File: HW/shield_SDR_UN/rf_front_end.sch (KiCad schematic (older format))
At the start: 73 parts, among them P1 GSG-RF-CONN, P2 GSG-RF-CONN, Q1 MOSFET_P, T1 BALUN, T2 BALUN, U1 MAX2830, U2 SI5351C, U3 MAX5864, X1 GSG-XTAL4PIN

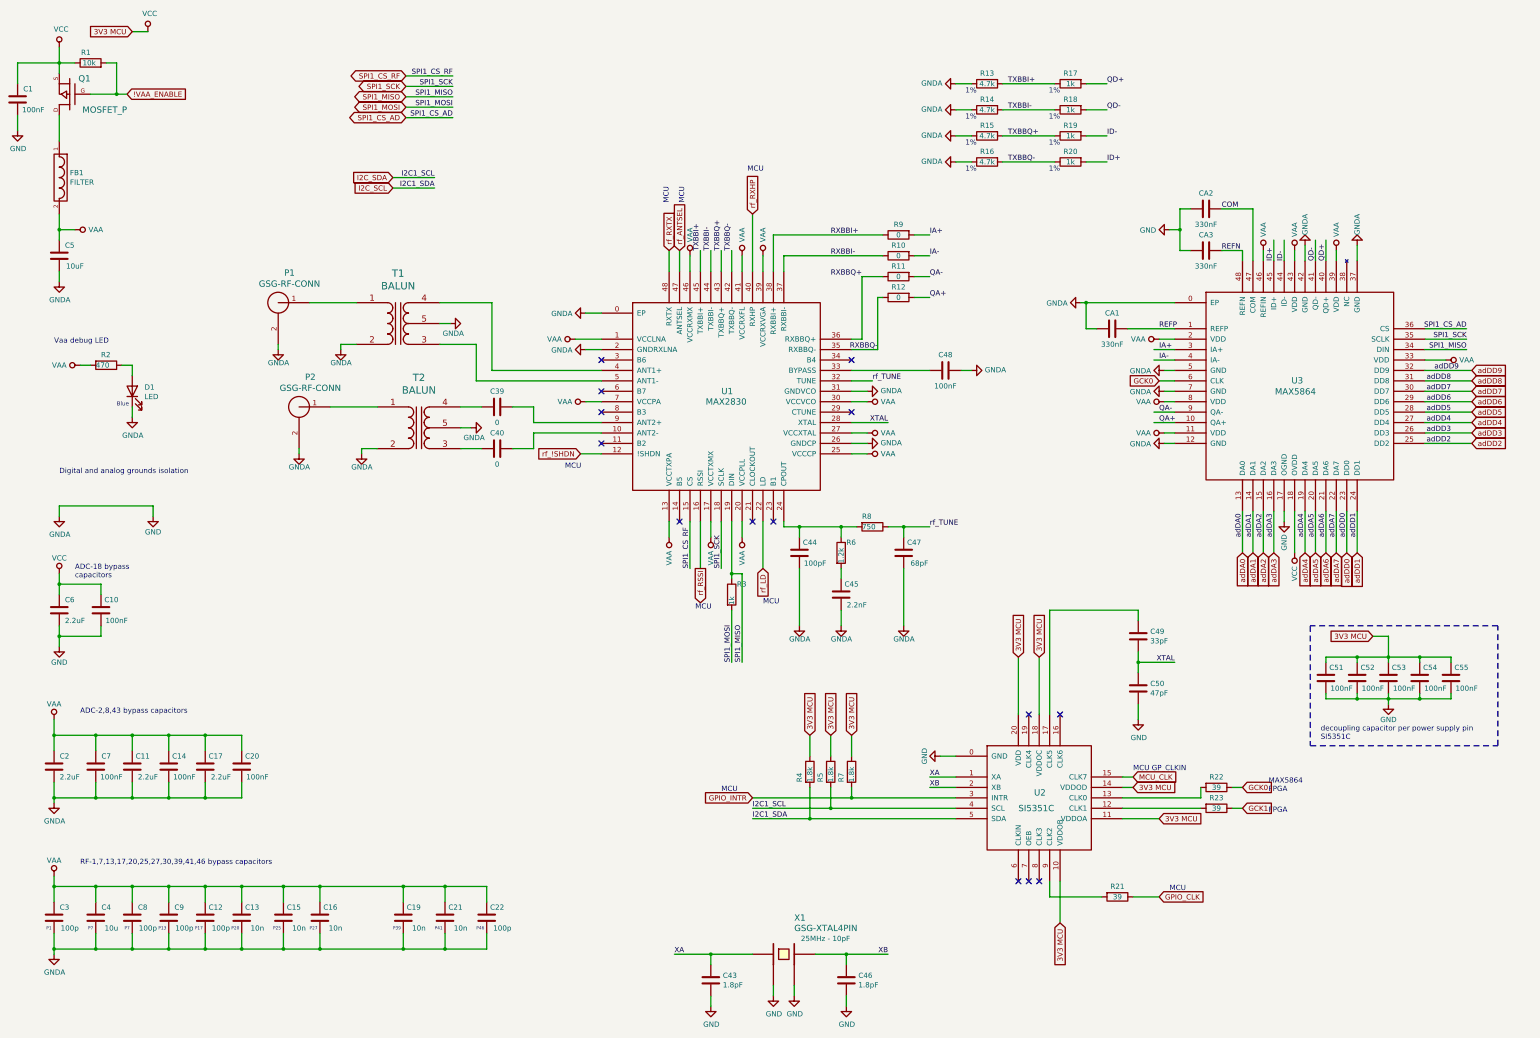
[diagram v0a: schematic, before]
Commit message: PCB route V4
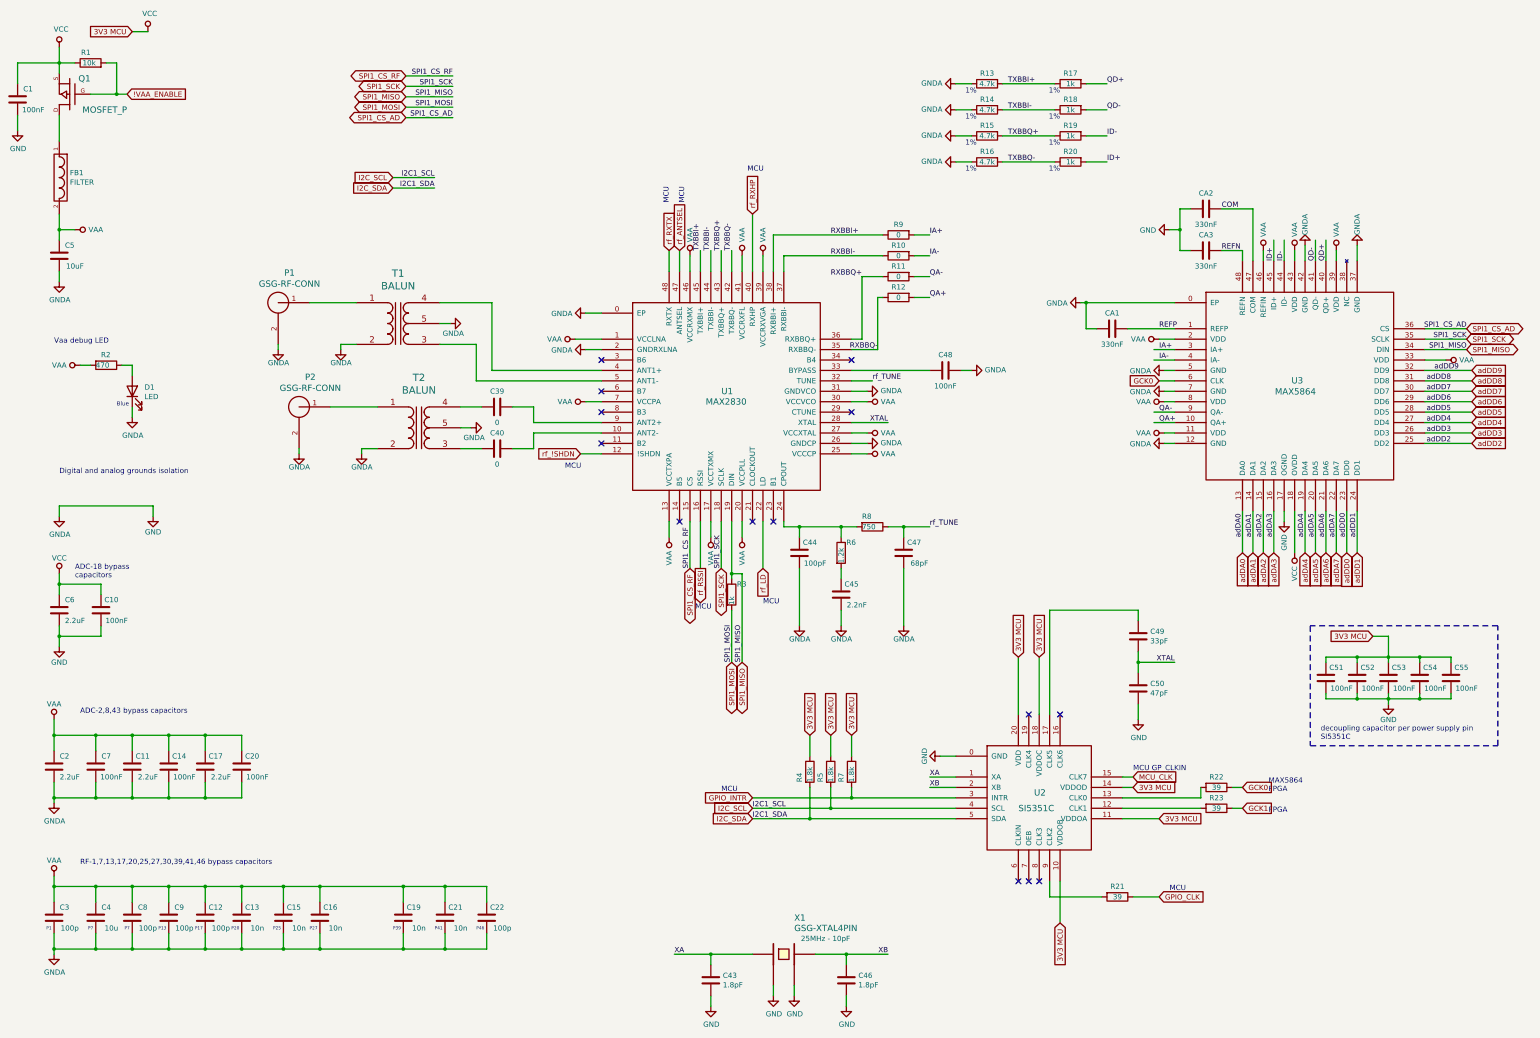
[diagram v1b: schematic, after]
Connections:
- net I2C_SCL: now also R5.2, U2.4 (SCL); no longer R4.2, U2.5 (SDA)
- net I2C_SDA: now also R4.2, U2.5 (SDA); no longer R5.2, U2.4 (SCL)
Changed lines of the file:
@@
 Text Label 4850 2200 2    50   ~ 0
 I2C1_SCL
-Text GLabel 4450 2300 0    50   Input ~ 0
+Text GLabel 7900 8250 0    50   Input ~ 0
 I2C_SCL
-Text GLabel 4450 2200 0    50   Input ~ 0
+Text GLabel 7900 8350 0    50   Input ~ 0
 I2C_SDA
 Wire Wire Line
@@
 Wire Wire Line
 	3750 9000 4550 9000
+Text GLabel 7300 5950 3    50   BiDi ~ 0
+SPI1_CS_RF
+Text GLabel 7800 6850 3    50   BiDi ~ 0
+SPI1_MISO
+Text GLabel 14750 3650 2    50   BiDi ~ 0
+SPI1_CS_AD
+Text GLabel 7700 6850 3    50   BiDi ~ 0
+SPI1_MOSI
+Text GLabel 7600 5950 3    50   BiDi ~ 0
+SPI1_SCK
+Text GLabel 14750 3850 2    50   BiDi ~ 0
+SPI1_MISO
+Text GLabel 14750 3750 2    50   BiDi ~ 0
+SPI1_SCK
+Text GLabel 4450 2200 0    50   Input ~ 0
+I2C_SCL
+Text GLabel 4450 2300 0    50   Input ~ 0
+I2C_SDA
 $EndSCHEMATC
